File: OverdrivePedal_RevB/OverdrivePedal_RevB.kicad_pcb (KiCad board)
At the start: 2 copper layers, 26.7 x 33.7 mm, 23 parts, among them J1 Conn_01x02, J2 Conn_01x02, J3 Conn_01x03, J4 Conn_01x03, J5 Conn_01x03, J6 Conn_01x02, U1 TL072, U2 NCP1729, U3 MIC5233-5.0YM5-TR, U4 MIC5270-5.0YM5-TR

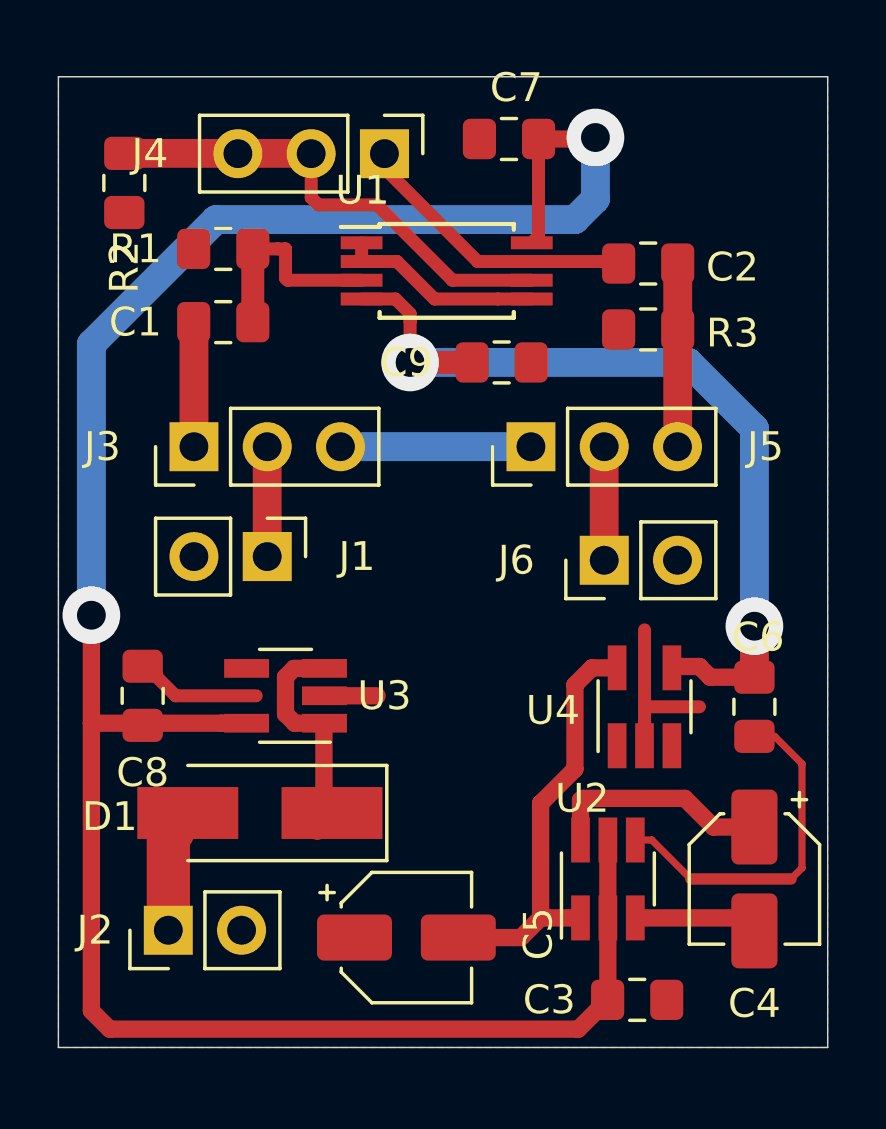
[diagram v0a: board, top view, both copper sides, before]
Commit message: modified RevB
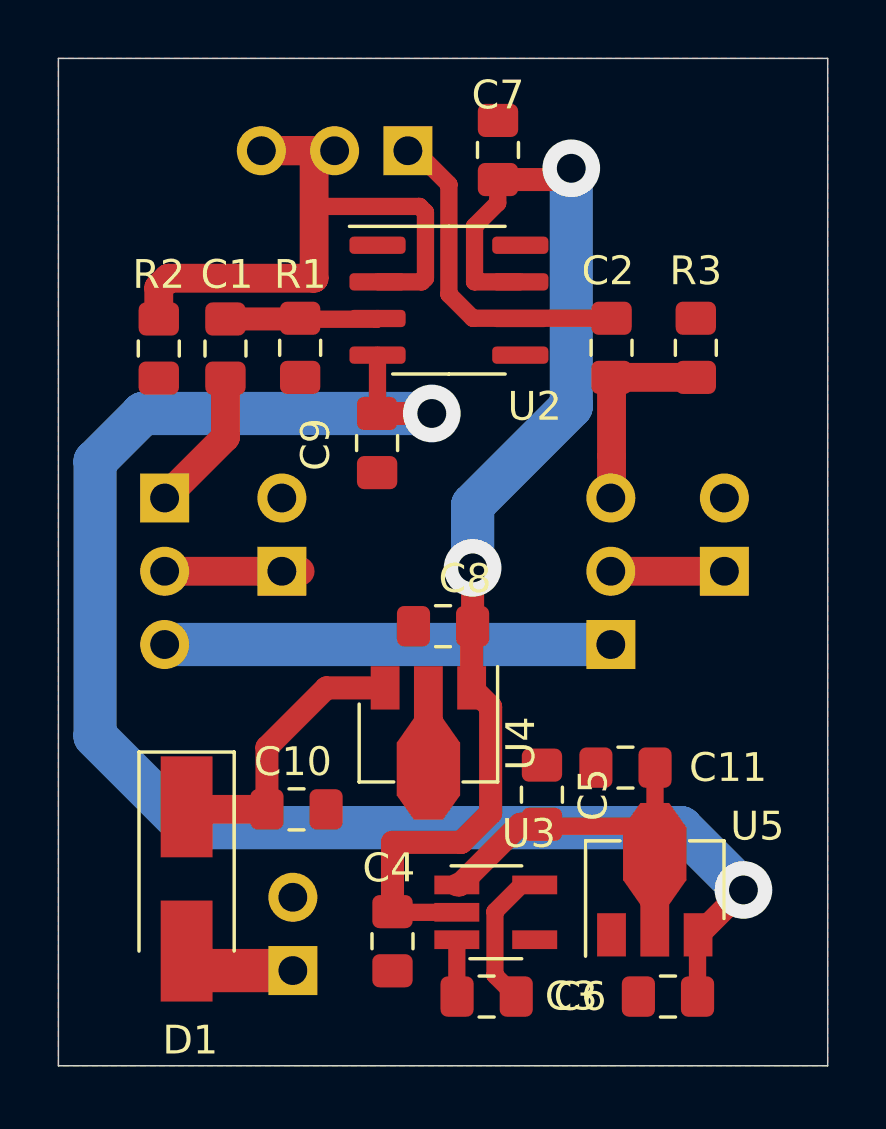
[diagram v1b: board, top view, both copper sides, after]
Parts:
- removed U1: TL072, Package_SO:TSSOP-8_4.4x3mm_P0.65mm
- added C10: 330nF, Capacitor_SMD:C_0805_2012Metric_Pad1.15x1.40mm_HandSolder, F.Cu at (67.3, 193.7)
- added C11: 1uF, Capacitor_SMD:C_0805_2012Metric_Pad1.15x1.40mm_HandSolder, F.Cu at (78.7, 192.2)
- added U5: XC6902N501PR-G, Package_TO_SOT_SMD:SOT-89-3, F.Cu at (79.7, 196.5)
- C3: value 100nF -> 1uF
- C4, C5: value 10uF -> 1uF; footprint Capacitor_SMD:CP_Elec_4x5.7 -> Capacitor_SMD:C_0805_2012Metric_Pad1.15x1.40mm_HandSolder
- C8: value 2.2uF -> 100nF
- J1, J2, J3, J4, J5, J6: moved to B.Cu
- U2: value NCP1729 -> TL071; footprint Package_TO_SOT_SMD:SOT-23-6_Handsoldering -> Package_SO:SOIC-8_3.9x4.9mm_P1.27mm
- U3: value MIC5233-5.0YM5-TR -> TPS60400
- U4: value MIC5270-5.0YM5-TR -> KIA78L05T; footprint Package_TO_SOT_SMD:SOT-23-5_HandSoldering -> Package_TO_SOT_SMD:SOT-89-3
- moved U2 20.8 mm to (72.6, 176.0), turned to 0 degrees
- moved C4 12.7 mm to (70.6, 198.2)
- moved C8 10.7 mm to (72.4, 187.3), turned to 180 degrees
- moved C6 10.5 mm to (80.2, 200.2), turned to 180 degrees
- moved U3 10.5 mm to (74.2, 197.2), turned to 0 degrees
- moved U4 7.54 mm to (71.9, 190.9), turned to 270 degrees
- moved J5 7.40 mm to (78.2, 188.0), turned to 0 degrees
- moved C5 6.83 mm to (75.8, 193.2), turned to 90 degrees
- moved R2 5.86 mm to (62.5, 177.7)
- moved C3 5.22 mm to (73.9, 200.2)
- moved C9 5.14 mm to (70.1, 181.0), turned to 270 degrees
- moved J2 4.54 mm to (67.2, 199.3), turned to 0 degrees
- moved R1 4.34 mm to (67.4, 177.7), turned to 270 degrees
- moved J6 4.18 mm to (82.1, 185.4), turned to 0 degrees
- moved D1 3.42 mm to (63.5, 196.1), turned to 270 degrees
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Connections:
- C3 pad 1: +5V -> Net-(C3-Pad1)
- C3 pad 2: GNDS -> Net-(C3-Pad2)
- C4 pad 1: Net-(C4-Pad1) -> +5V
- C4 pad 2: Net-(C4-Pad2) -> GNDS
- C5 pad 1: GNDS -> /PosNeg5V_PSU/-5V_POL
- C5 pad 2: /PosNeg5V_PSU/-5V_POL -> GNDS
- U2 pad 1: /PosNeg5V_PSU/-5V_POL -> Net-(U2-Pad1)
- U2 pad 2: +5V -> Net-(J4-Pad2)
- U2 pad 3: Net-(C4-Pad2) -> Net-(C1-Pad1)
- U2 pad 4: GNDS -> -5V
- U2 pad 5: +5V -> Net-(U2-Pad5)
- U2 pad 6: Net-(C4-Pad1) -> Net-(C2-Pad2)
- U3 pad 1: /PosNeg5V_PSU/+9V_POL -> /PosNeg5V_PSU/-5V_POL
- U3 pad 2: GNDS -> +5V
- U3 pad 3: /PosNeg5V_PSU/+9V_POL -> Net-(C3-Pad1)
- U3 pad 4: Net-(U3-Pad4) -> GNDS
- U3 pad 5: +5V -> Net-(C3-Pad2)
- U4 pad 1: Net-(U4-Pad1) -> +5V
- U4 pad 3: Net-(U4-Pad3) -> /PosNeg5V_PSU/+9V_POL
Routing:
- net +5V: track 80.1 -> 40.6 mm
- net GNDS: track 24.8 -> 0.00 mm
- net -5V: track 30.3 -> 54.9 mm
- net Net-(J3-Pad3): track 6.60 -> 15.5 mm
- net Net-(C4-Pad1): track 7.85 -> 0.00 mm
- net Net-(U1-Pad1): track 7.09 -> 0.00 mm
- net Net-(J4-Pad2): track 16.8 -> 23.3 mm
- net Net-(C3-Pad2): track 0.00 -> 5.01 mm
- net Net-(C4-Pad2): track 4.32 -> 0.00 mm
- net /PosNeg5V_PSU/+9V_POL: track 7.85 -> 11.4 mm
- net Net-(C1-Pad1): track 7.36 -> 5.31 mm
- net Net-(C3-Pad1): track 0.00 -> 1.97 mm
- net Net-(C2-Pad2): track 9.99 -> 11.7 mm
- net /PosNeg5V_PSU/-5V_POL: track 14.8 -> 13.6 mm
- net Net-(C1-Pad2): track 4.19 -> 5.03 mm
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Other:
- board size 26.7 x 33.7 mm -> 26.7 x 34.9 mm
